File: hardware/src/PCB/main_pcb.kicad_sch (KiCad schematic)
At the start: 44 parts, among them J1 Batt, J2 Hall_sensor, J3 Pressure_sensor, Q1 BSS138, Q2 BSS138, Q3 BSS138, SW1 Button, SW2 Button, U2 XIAO-nRF52840-Plus-SMD

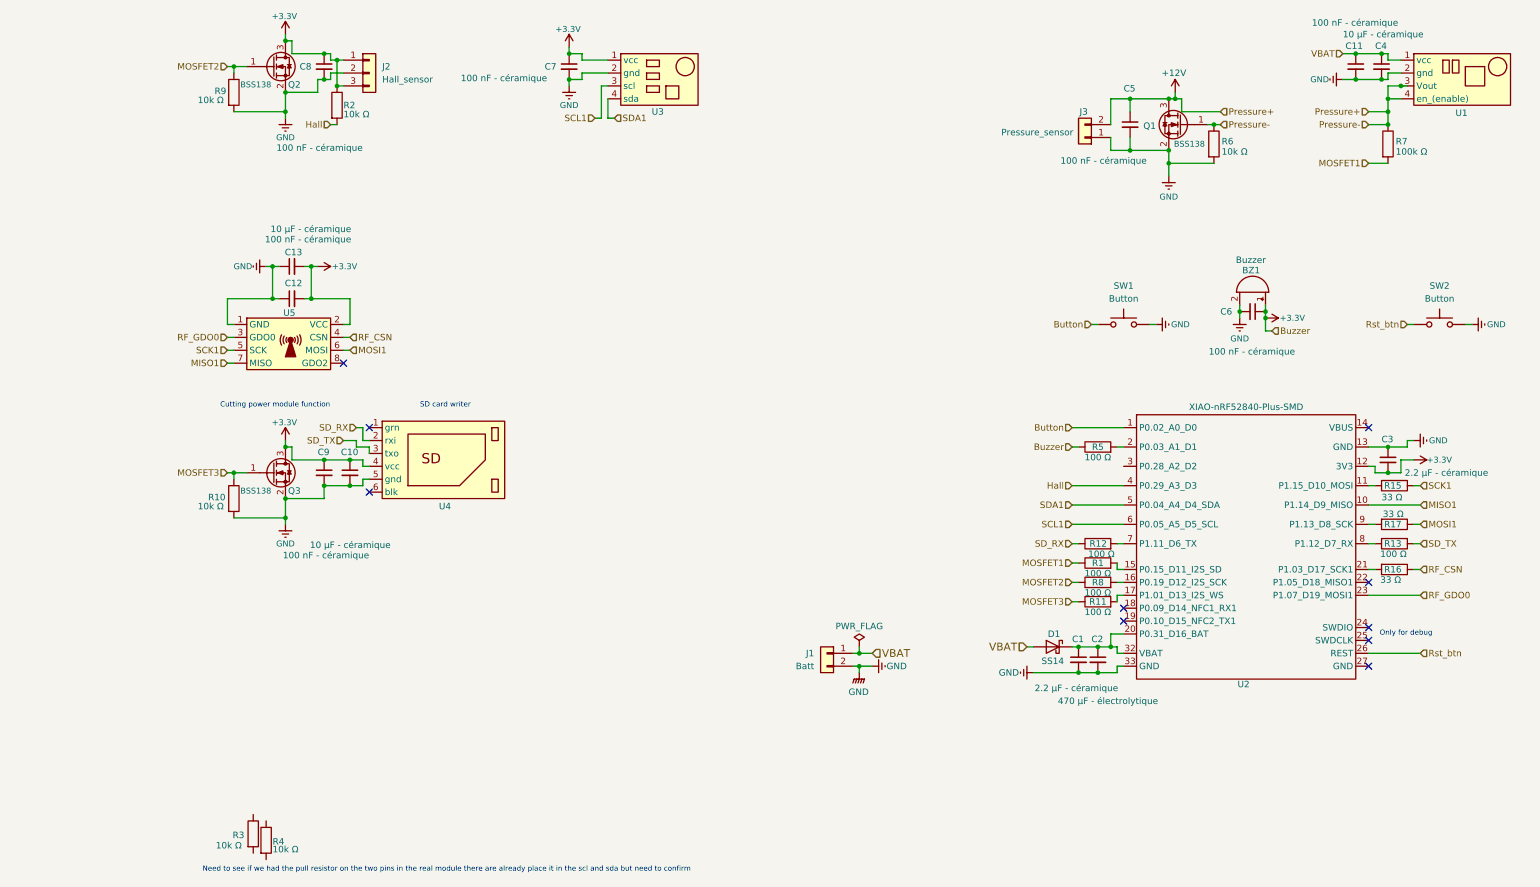
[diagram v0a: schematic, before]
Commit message: feature: PCB advancement
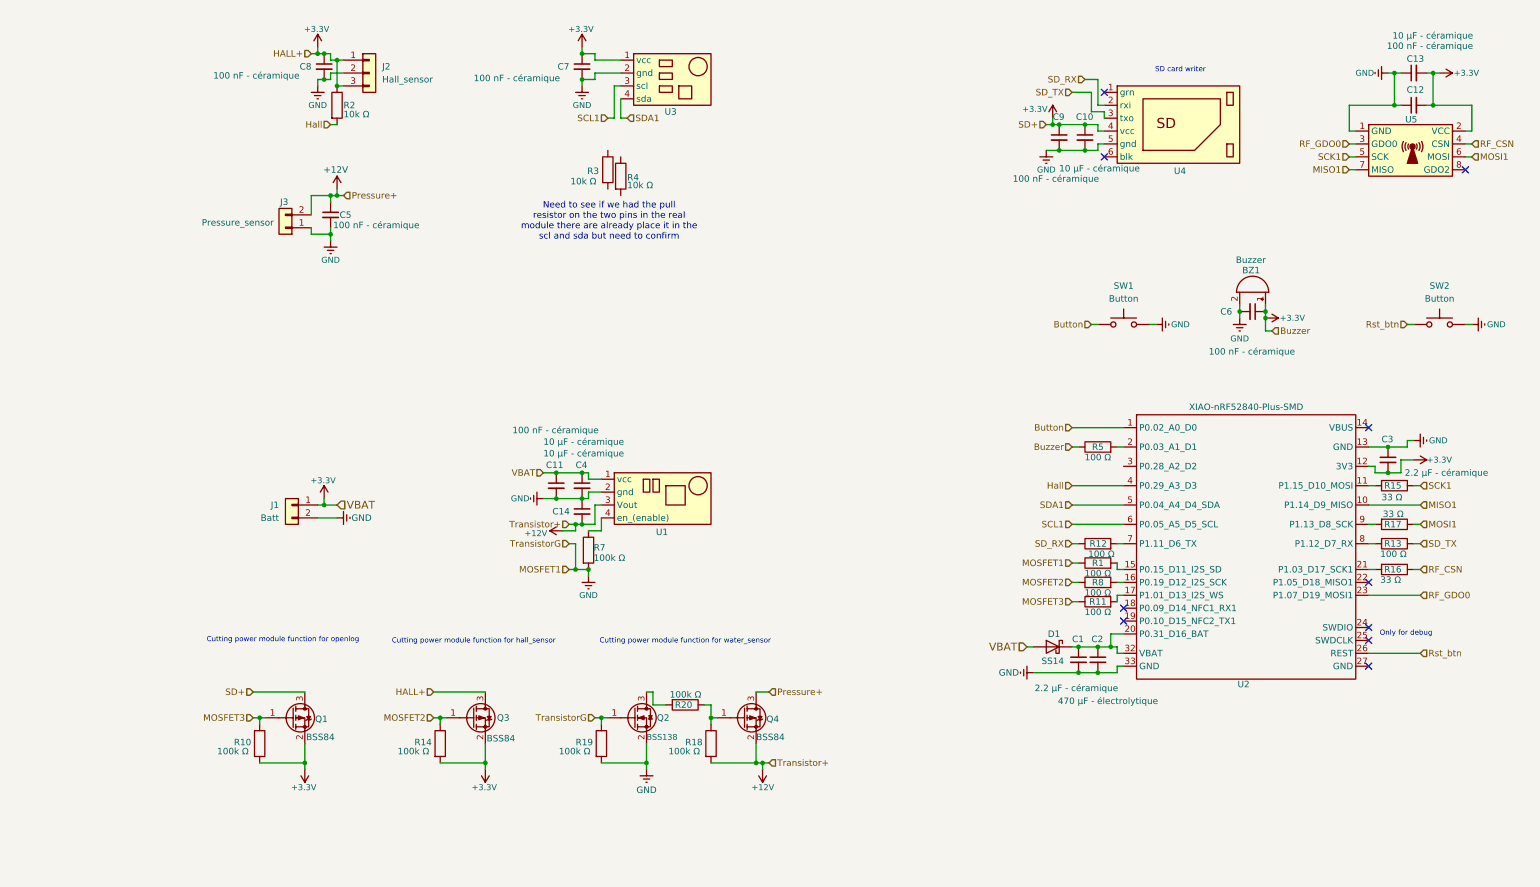
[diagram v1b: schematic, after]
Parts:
- removed Q1, Q3: BSS138, Package_TO_SOT_SMD:SOT-23, symbol Transistor_FET:BSS138
- removed R6, R9: 10k Ω, Resistor_SMD:R_0201_0603Metric, symbol Device:R
- added C14: 10 µF - céramique, Capacitor_SMD:C_0603_1608Metric, symbol Device:C_Small
- added Q1, Q3, Q4: BSS84, Package_TO_SOT_SMD:SOT-23, symbol Transistor_FET:BSS84
- added R14, R18, R19, R20: 100k Ω, Resistor_SMD:R_0201_0603Metric, symbol Device:R
- R10: value 10k Ω -> 100k Ω
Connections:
- net MOSFET1 is gone; now on net GND: R1.1, R7.2
- net VBAT is gone; now on net +3.3V: C11.1, C4.1, D1.2 (A), J1.1 (Pin_1), U1.1 (vcc)
- net +12V: now also C14.2, Q4.2 (S), Q4.3 (D), R18.2; no longer R7.1, U1.4 (en_(enable))
- net +3.3V: now also R10.2, Q1.2 (S), Q1.3 (D), Q3.2 (S), Q3.3 (D), R14.2; no longer Q2.3 (D)
- net GND: now also Q2.1 (G), C14.1, R19.1, R19.2; no longer R10.2
- net MOSFET2: now also Q3.1 (G), R14.1; no longer Q2.1 (G)
- net MOSFET3: now also Q1.1 (G)
- new net: R7.1, U1.4 (en_(enable))
- new net: Q2.3 (D), R20.2
- new net: Q4.1 (G), R18.1, R20.1
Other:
- note added: "Need to see if we had the pull resistor on the two pins in the real module there are already place it in the scl and sda but need to confirm"
- note added: "^{Cutting power module function for hall_sensor}"
- note added: "^{Cutting power module function for openlog}"
- note added: "^{Cutting power module function for water_sensor}"
- note removed: "^{Cutting power module function}"
- note removed: "^{Need to see if we had the pull resistor on the two pins in the real module there are already place it in the scl and sda but need to confirm}"
- moved on the sheet: C10, C11, C12, C13, C4, C5, C7, C9, J1, J3, R10, R3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
